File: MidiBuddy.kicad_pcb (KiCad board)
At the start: 2 copper layers, 3 parts, among them J1 DIN-5, J2 DIN-5, U1 6N136

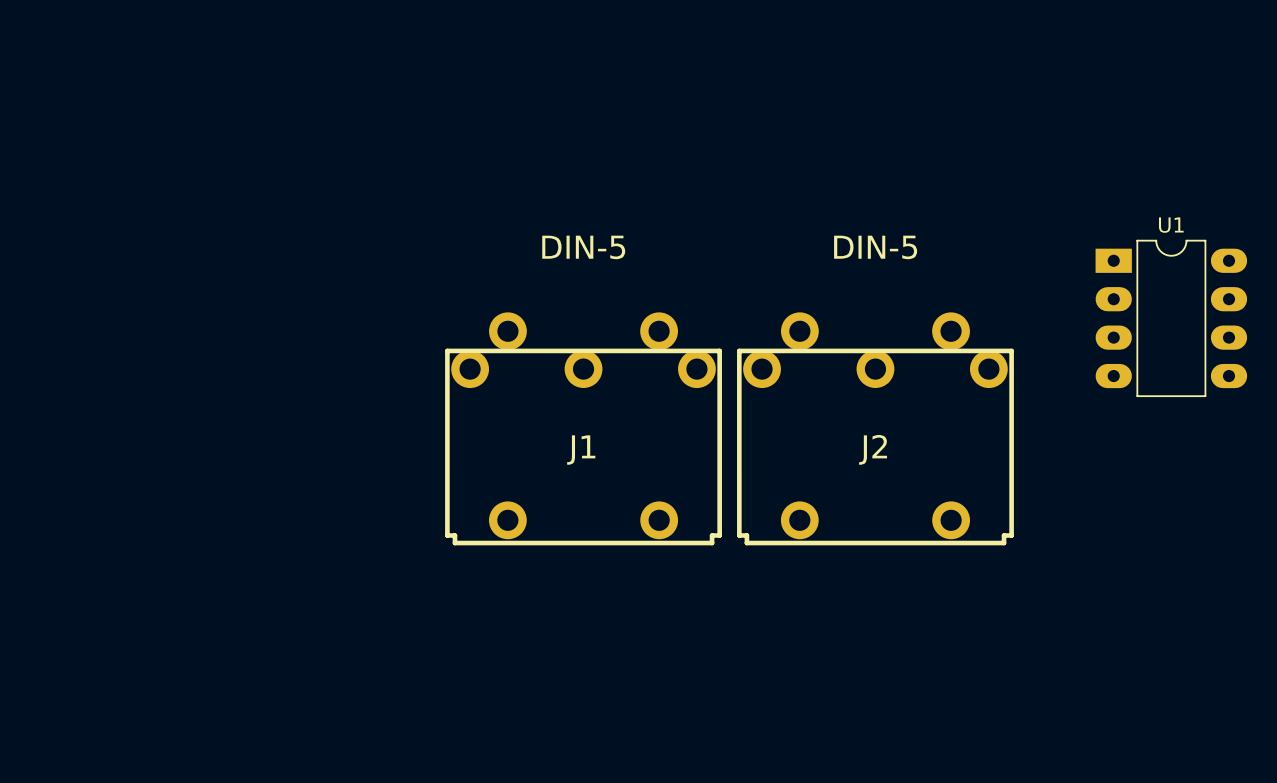
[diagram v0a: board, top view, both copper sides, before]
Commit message: Initial pcb design
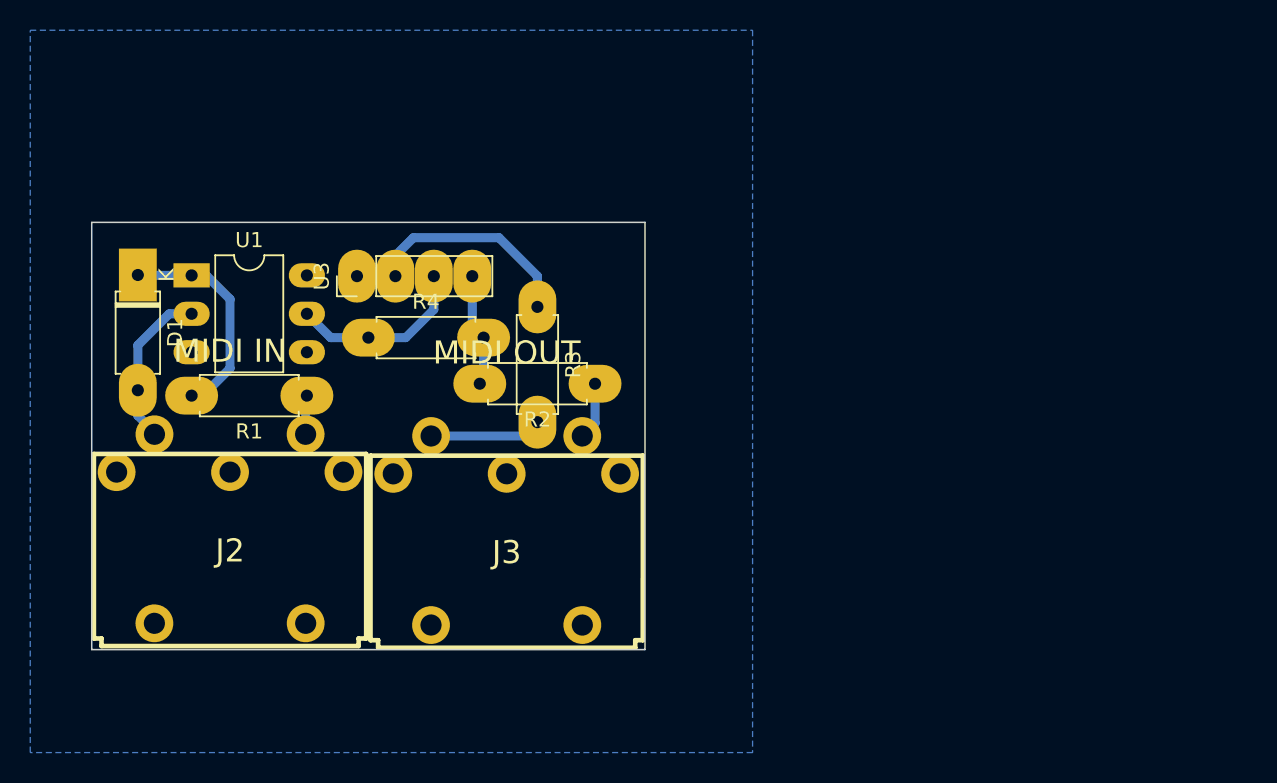
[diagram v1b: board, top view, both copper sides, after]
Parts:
- removed J1: DIN-5, midi:midi
- added D1: 1N1418, Diode_THT:D_A-405_P7.62mm_Horizontal, F.Cu at (76.2, 73.1)
- added J3: MIDI OUT, midi:midi, F.Cu at (100.6, 89.2)
- added R1: 220, Resistor_THT:R_Axial_DIN0207_L6.3mm_D2.5mm_P7.62mm_Horizontal, F.Cu at (87.4, 81.1)
- added R2: 1k, Resistor_THT:R_Axial_DIN0207_L6.3mm_D2.5mm_P7.62mm_Horizontal, F.Cu at (106.4, 80.3)
- added R3: 220, Resistor_THT:R_Axial_DIN0207_L6.3mm_D2.5mm_P7.62mm_Horizontal, F.Cu at (102.6, 75.2)
- added R4: 1k, Resistor_THT:R_Axial_DIN0207_L6.3mm_D2.5mm_P7.62mm_Horizontal, F.Cu at (91.4, 77.2)
- added U3: TTL, Connector_PinHeader_2.54mm:PinHeader_1x04_P2.54mm_Vertical, F.Cu at (90.7, 73.2)
- J2: value DIN-5 -> MIDI IN
- U1: value 6N136 -> 4N35; footprint Package_DIP:DIP-8_W7.62mm_LongPads -> Package_DIP:DIP-6_W7.62mm_LongPads
- moved U1 61.0 mm to (79.8, 73.1)
- moved J2 43.2 mm to (82.3, 89.1)
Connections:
- J2 pad 4: unconnected-(J2-Pad4) -> Net-(J2-Pad4)
- J2 pad 5: unconnected-(J2-Pad5) -> Net-(D1-Pad2)
- U1 pad 1: unconnected-(U1-Pad1) -> Net-(D1-Pad1)
- U1 pad 2: unconnected-(U1-Pad2) -> Net-(D1-Pad2)
- U1 pad 4: unconnected-(U1-Pad4) -> GND
- U1 pad 5: unconnected-(U1-Pad5) -> /RX
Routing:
- net Net-(D1-Pad1): track 0.00 -> 14.6 mm
- net /TX: track 0.00 -> 14.3 mm
- net /RX: track 0.00 -> 12.0 mm
- net Net-(D1-Pad2): track 0.00 -> 10.8 mm
- net +3V3: track 0.00 -> 7.53 mm
- net Net-(J3-Pad5): track 0.00 -> 7.41 mm
- net Net-(J3-Pad4): track 0.00 -> 3.81 mm
- net Net-(J2-Pad4): track 0.00 -> 2.59 mm
- added copper zone on B.Cu, net GND
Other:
- board outline added: 36.6 x 28.2 mm

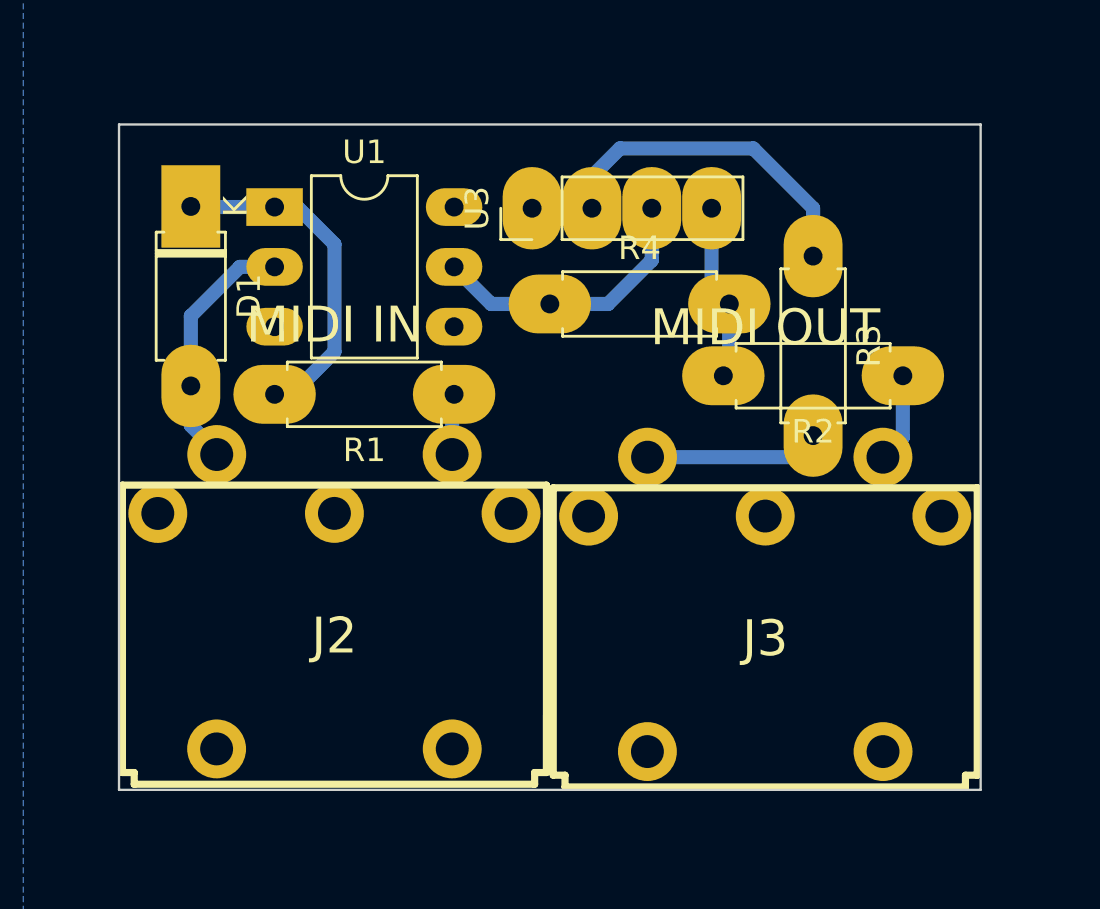
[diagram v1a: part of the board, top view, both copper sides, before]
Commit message: Minor adjustments
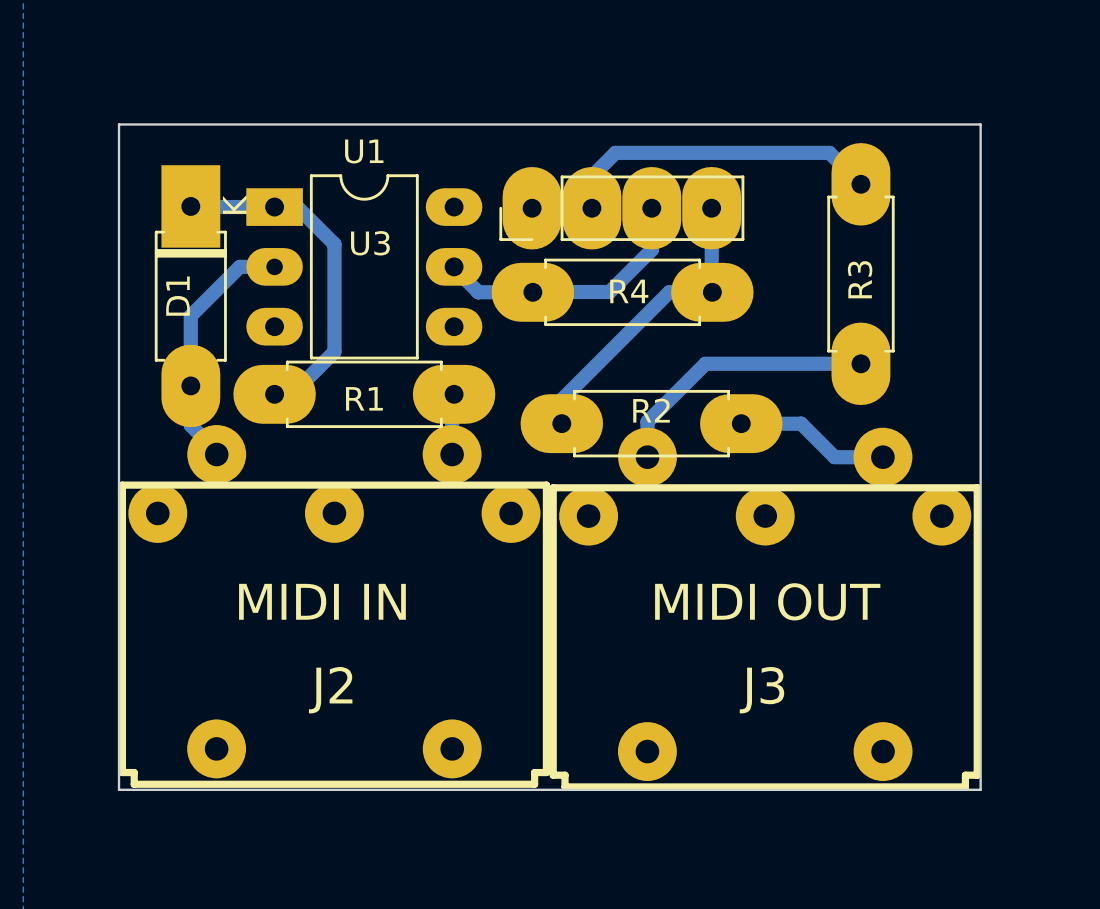
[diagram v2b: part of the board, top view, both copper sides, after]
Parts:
- moved R2 7.15 mm to (99.6, 82.3)
- moved R3 3.66 mm to (104.6, 72.1)
- moved R4 0.87 mm to (90.7, 76.7)
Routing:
- net +3V3: track 7.53 -> 12.9 mm
- net Net-(J3-Pad5): track 7.41 -> 11.6 mm
- net Net-(J3-Pad4): track 3.81 -> 6.60 mm
- net /RX: track 12.0 -> 11.4 mm
- net /TX: track 14.3 -> 13.7 mm
